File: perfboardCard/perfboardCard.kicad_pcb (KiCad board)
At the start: 2 copper layers, 39.9 x 8.5 mm, 2 parts, among them J1 Conn_02x20_Top_Bottom, J2 Conn_02x19_Top_Bottom

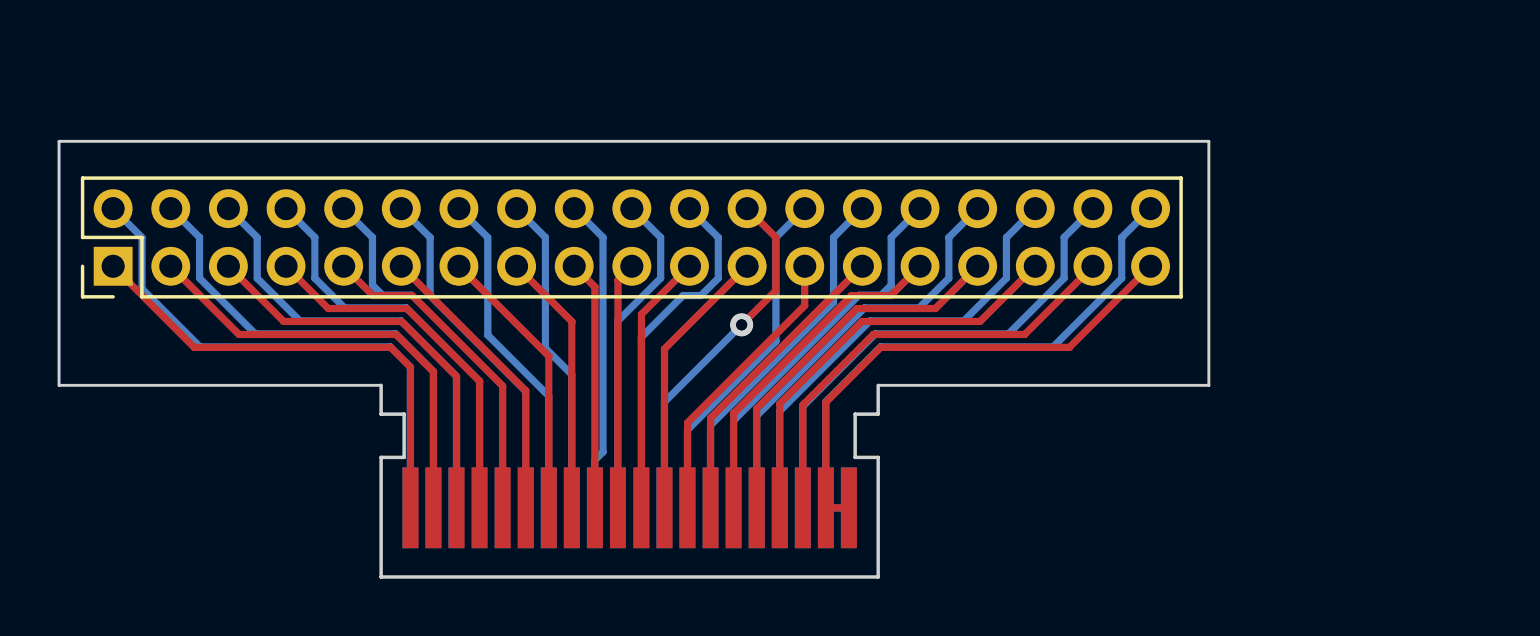
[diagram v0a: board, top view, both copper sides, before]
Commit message: Board revision 1
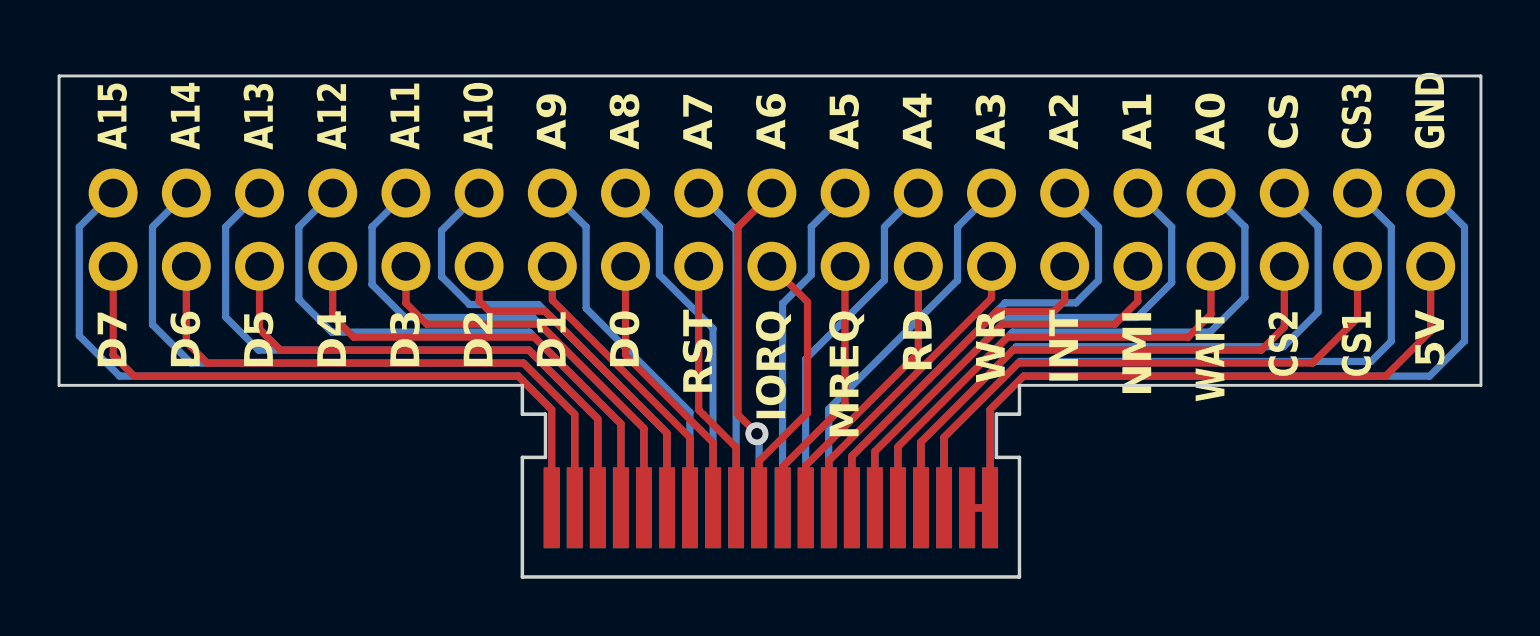
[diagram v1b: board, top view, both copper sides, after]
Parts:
- J2: footprint Connector_PinHeader_2.00mm:PinHeader_2x19_P2.00mm_Vertical -> Connector_PinHeader_2.54mm:PinHeader_2x19_P2.54mm_Vertical
- moved J1 4.90 mm to (104.9, 103.4)
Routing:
- net GND: track 19.4 -> 27.3 mm
- net /A15: track 18.5 -> 26.3 mm
- net /IO-CS3: track 17.3 -> 25.0 mm
- net /A14: track 17.0 -> 24.2 mm
- net /CS: track 16.0 -> 22.5 mm
- net /A13: track 15.7 -> 22.3 mm
- net /D7: track 16.7 -> 22.5 mm
- net /A0: track 14.7 -> 20.4 mm
- net /A12: track 14.4 -> 20.1 mm
- net +5V: track 17.7 -> 22.9 mm
- net /D6: track 15.4 -> 20.4 mm
- net /A1: track 13.5 -> 18.3 mm
- net /IO-CS1: track 15.6 -> 20.3 mm
- net /A11: track 13.3 -> 17.9 mm
- net /D5: track 14.1 -> 18.3 mm
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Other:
- board size 39.9 x 8.5 mm -> 49.3 x 10.7 mm
- board text added: "5V"
- board text added: "A0"
- board text added: "A1"
- board text added: "A10"
- board text added: "A11"
- board text added: "A12"
- board text added: "A13"
- board text added: "A14"
- board text added: "A15"
- board text added: "A2"
- board text added: "A3"
- board text added: "A4"
- board text added: "A5"
- board text added: "A6"
- board text added: "A7"
- board text added: "A8"
- board text added: "A9"
- board text added: "CS"
- board text added: "CS1"
- board text added: "CS2"
- board text added: "CS3"
- board text added: "D0"
- board text added: "D1"
- board text added: "D2"
- board text added: "D3"
- board text added: "D4"
- board text added: "D5"
- board text added: "D6"
- board text added: "D7"
- board text added: "GND"
- board text added: "INT"
- board text added: "IORQ"
- board text added: "MREQ"
- board text added: "NMI"
- board text added: "RD"
- board text added: "RST"
- board text added: "WAIT"
- board text added: "WR"
